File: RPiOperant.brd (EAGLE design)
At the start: 80 x 64 mm, 34 parts, among them IC1 74LS14N, IC3 MCP3008, J2 POWER_JACK, J3 POWER_JACK

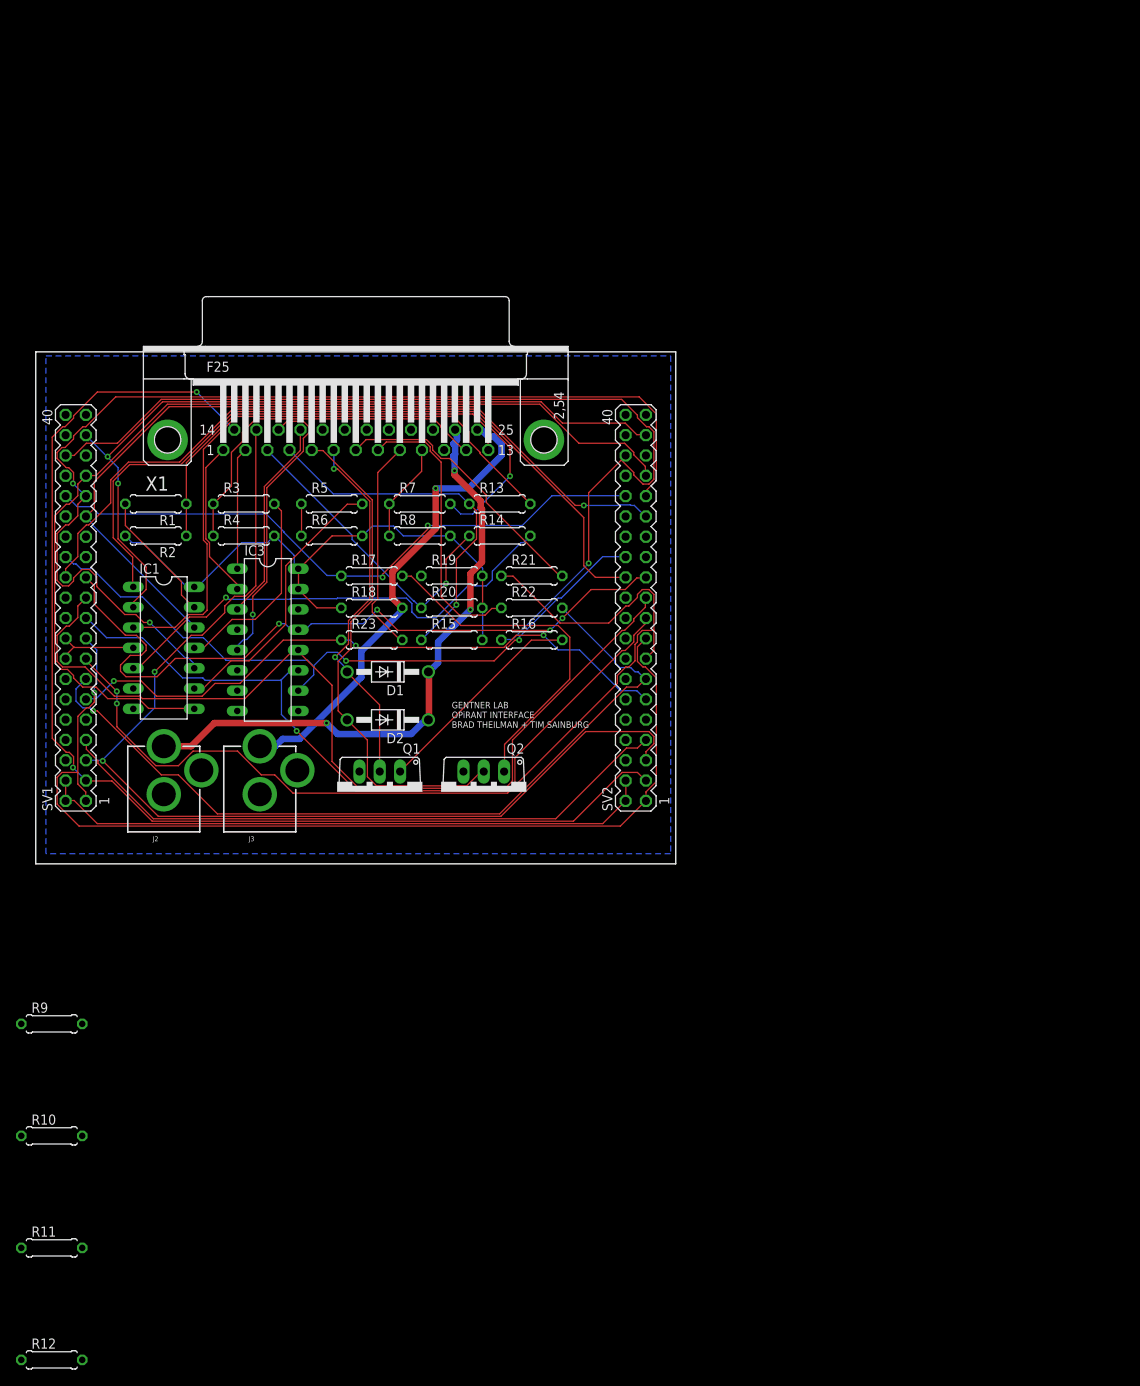
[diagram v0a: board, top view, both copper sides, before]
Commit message: new board
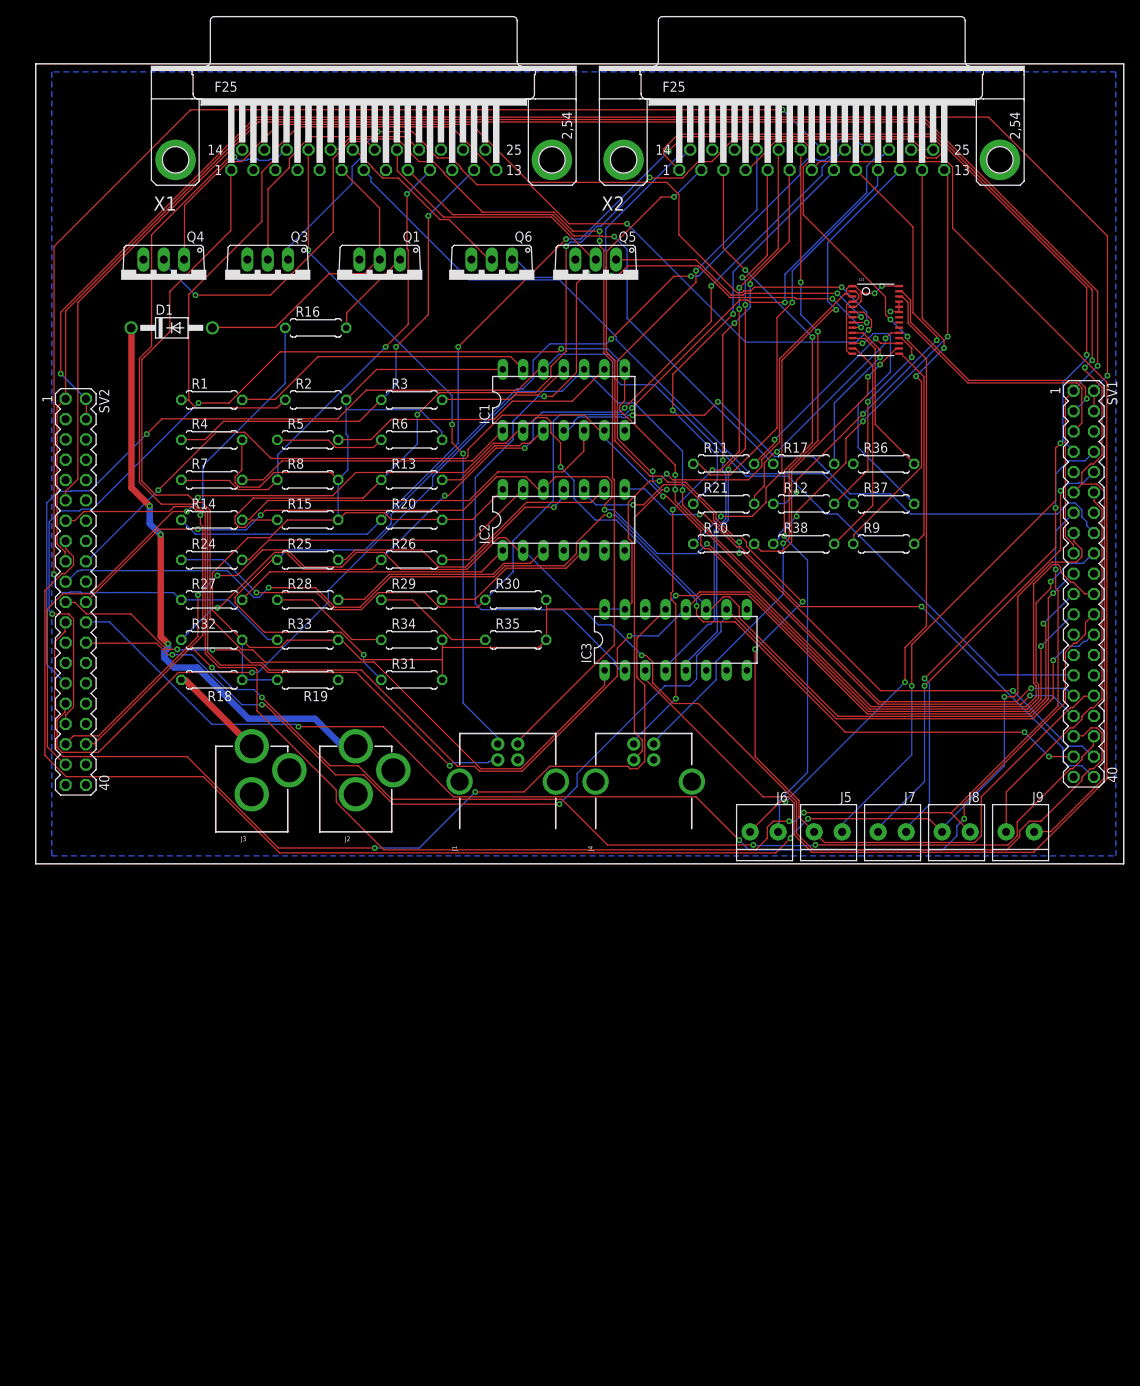
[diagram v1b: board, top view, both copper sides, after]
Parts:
- removed D2: 1N4004, diode:DO41-10
- removed Q2: (no value), adafruit:TO220V
- removed R22, R23: 330, resistor:0207/7
- added IC2: 74LS14N, 74xx-us:DIL14
- added J1, J4: USB_B_PTH, SparkFun-Connectors:USB-B-PTH
- added J5, J6, J7, J8, J9: 1X2-3.5MM, adafruit:1X2-3.5MM
- added Q3, Q4, Q5, Q6: (no value), adafruit:TO220V
- added R24, R25, R26, R27, R28, R29: 1k, resistor:0207/7
- added R30, R31, R32, R33, R34, R35: 4.3k, resistor:0207/7
- added R36, R37, R38: 330, resistor:0207/7
- added U1: (no value), adafruit:TSSOP28
- added X2: (no value), con-subd:F25HP
- R17: value 1k -> 330
- moved R12 142.4 mm to (96.0, 45.0)
- moved R11 129.1 mm to (86.0, 50.0)
- moved SV1 126.0 mm to (131.0, 35.0), turned to 270 degrees
- moved R9 120.1 mm to (106.0, 40.0)
- moved R10 111.9 mm to (86.0, 40.0)
- moved SV2 70.0 mm to (5.00, 34.0), turned to 270 degrees
- moved Q1 64.0 mm to (43.0, 73.0)
- moved IC1 58.8 mm to (66.0, 58.0), turned to 0 degrees
- moved R17 55.8 mm to (96.0, 50.0)
- moved IC3 51.0 mm to (80.0, 28.0), turned to 0 degrees
- moved D1 50.8 mm to (17.0, 67.0), turned to 0 degrees
- moved R16 47.4 mm to (35.0, 67.0)
- moved R14 36.1 mm to (22.0, 43.0)
- moved X1 35.0 mm to (41.0, 88.0)
- moved R2 26.2 mm to (35.0, 58.0), turned to 0 degrees
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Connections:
- removed net GPIO2: SV1.3, SV2.3, X1.14
- removed net GPIO25: X1.18
- removed net GPIO3: SV1.5, SV2.5, X1.15
- removed net GPIO4: SV1.7, SV2.7
- removed net HOPPER_IR_LED: R12.1, X1.19
- removed net HOUSE_LIGHTS: D2.A, Q2.2, X1.5
- removed net IR_LED_C: R10.1, X1.21
- removed net IR_LED_L: R9.1, X1.22
- removed net IR_LED_R: R11.1, X1.20
- removed net LIGHTS_TRIG_GPIO: R17.1, SV1.32, SV2.32
- new net AUX1: J5.1, SV1.7, X2.1
- new net AUX2: J5.2, SV1.32, X2.2
- new net AUX3: J6.1, X2.3
- new net AUX4: J6.2, X2.4
- new net CENTNER_LED: R36.1
- new net GPIO18: J9.2, SV1.12
- new net HOUSELIGHT_B: Q4.2, X1.20
- new net HOUSELIGHT_B_GPIO: Q4.1, U1.8
- new net HOUSELIGHT_G: Q5.2, X1.21
- new net HOUSELIGHT_G_GPIO: Q5.1, U1.7
- new net HOUSELIGHT_R: Q3.2, X1.22
- new net HOUSELIGHT_R_GPIO: Q3.1, U1.6
- new net HOUSELIGHT_W: Q6.2, X1.19
- new net HOUSELIGHT_W_GPIO: Q6.1, U1.9
- new net IR_3: R24.1, R30.1, X2.23
- new net IR_3_GPIO: IC2.12, SV1.22, SV2.22
- new net IR_4: R25.1, R31.1, X2.22
- new net IR_4_GPIO: IC2.10, SV1.38
- new net IR_5: R26.1, R32.1, X2.21
- new net IR_5_GPIO: IC2.8, SV1.40
- new net IR_6: R27.1, R33.1, X2.20
- new net IR_6_GPIO: IC2.2, SV1.35, SV2.35
- new net IR_7: R28.1, R34.1
- new net IR_8: R29.1, R35.1
- new net LED_1: R38.1, X2.13
- new net LED_2: R9.1, X2.12
- new net LED_3: R10.1, X2.11
- new net LED_4: R11.1, X2.10
- new net LED_5: R12.1, X2.9
- new net LED_6: R21.1, X2.8
- new net LOADCELL2A+: X2.16
- new net LOADCELL2A-: X2.15
- new net LOADCELLA+: X1.15
- new net LOADCELLA-: X1.14
- new net LOADCELLE+: X1.25
- new net LOADCELLE-: X1.24
- new net N$11: IC2.5, R29.2
- new net N$13: R17.2, U1.10
- new net N$14: R36.2, U1.11
- new net N$15: R37.2, U1.12
- new net N$16: R38.2, U1.13
- new net N$17: IC2.4
- new net N$18: IC2.6
- new net N$26: R9.2, U1.15
- new net N$28: R11.2, U1.17
- new net N$29: R12.2, U1.18
- new net N$3: IC2.13, R24.2
- new net N$30: R21.2, U1.19
- new net N$4: IC2.11, R25.2
- new net N$5: IC2.9, R26.2
- new net N$7: IC2.1, R27.2
- new net N$9: IC2.3, R28.2
- new net RGB_CUE_B: X1.4
- new net RGB_CUE_G: X1.3
- new net RGB_CUE_R: X1.5
- new net RXD: J7.2, SV1.10
- new net SCL: SV1.5, U1.26
- new net SDA: SV1.3, U1.27
- new net TEMP: X1.2
- new net TXD: J7.1, SV1.8
- new net USB1_D+: J1.D+, X1.16
- new net USB1_D-: J1.D-, X1.17
- new net USB1_VBUS: J1.VBUS, X1.18
- new net USB2_D+: J4.D+, X2.17
- new net USB2_D-: J4.D-, X2.18
- new net USB2_VBUS: J4.VBUS, X2.19
- net +3V3: now also IC2.14, R30.2, R31.2, R32.2, R33.2, R34.2, R35.2, U1.1, U1.28, U1.3, U1.5; no longer R10.2, R11.2, R12.2, R9.2
- net +5V: no longer X1.25
- net 12V: no longer D2.C, X1.24
- net ADC0: now also X1.1; no longer X1.2
- net ADC1: now also X2.14; no longer X1.1
- net ADC2: now also X2.7; no longer X1.17
- net ADC3: now also X2.6
- net ADC4: now also X2.5; no longer X1.16
- net CENTER_LED: no longer R22.1
- net GND: now also IC2.7, J1.GND, J1.SHLD1, J1.SHLD2, J4.GND, J4.SHLD1, J4.SHLD2, Q3.3, Q4.3, Q5.3, Q6.3, U1.14, U1.2, U1.23, U1.24, U1.25, U1.4, X2.G1, X2.G2; no longer Q2.3
- net GPIO17: now also J9.1; no longer R23.1
- net GPIO22: now also J8.2; no longer R21.1
- net GPIO27: now also J8.1; no longer R22.2
- net IR_1: now also X2.25; no longer X1.4
- net IR_2: now also X2.24; no longer X1.3
- net LEFT_LED: now also R17.1; no longer R23.2
- net N$27: now also R10.2, U1.16; no longer Q2.1, R17.2
- net RIGHT_LED: now also R37.1; no longer R21.2
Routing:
- net +3V3: track 74.8 -> 262.4 mm, vias 0 -> 4
- net IR_6_GPIO: track 0.00 -> 179.9 mm, vias 0 -> 3
- net IR_6: track 0.00 -> 178.5 mm, vias 0 -> 2
- net GPIO17: track 79.0 -> 249.1 mm, vias 3 -> 2
- net IR_2_GPIO: track 0.00 -> 169.5 mm, vias 0 -> 3
- net IR_3_GPIO: track 0.00 -> 168.1 mm, vias 0 -> 4
- net AUX2: track 0.00 -> 153.0 mm, vias 0 -> 3
- net ADC2: track 25.7 -> 176.7 mm
- net AUX1: track 0.00 -> 147.7 mm, vias 0 -> 3
- net GPIO2: track 147.2 -> 0.00 mm, vias 2 -> 0
- net GPIO3: track 132.9 -> 0.00 mm, vias 2 -> 0
- net IR_4: track 0.00 -> 130.2 mm, vias 0 -> 3
- net IR_3: track 0.00 -> 128.7 mm, vias 0 -> 3
- net USB1_D+: track 0.00 -> 123.4 mm, vias 0 -> 2
- net ADC0: track 15.3 -> 130.4 mm
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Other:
- board size 80 x 64 mm -> 136 x 100 mm
- board text removed: "GENTNER LAB OPiRANT INTERFACE BRAD THEILMAN + TIM SAINBURG"
